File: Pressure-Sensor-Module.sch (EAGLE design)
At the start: 18 parts, among them IC1 ATTINY85

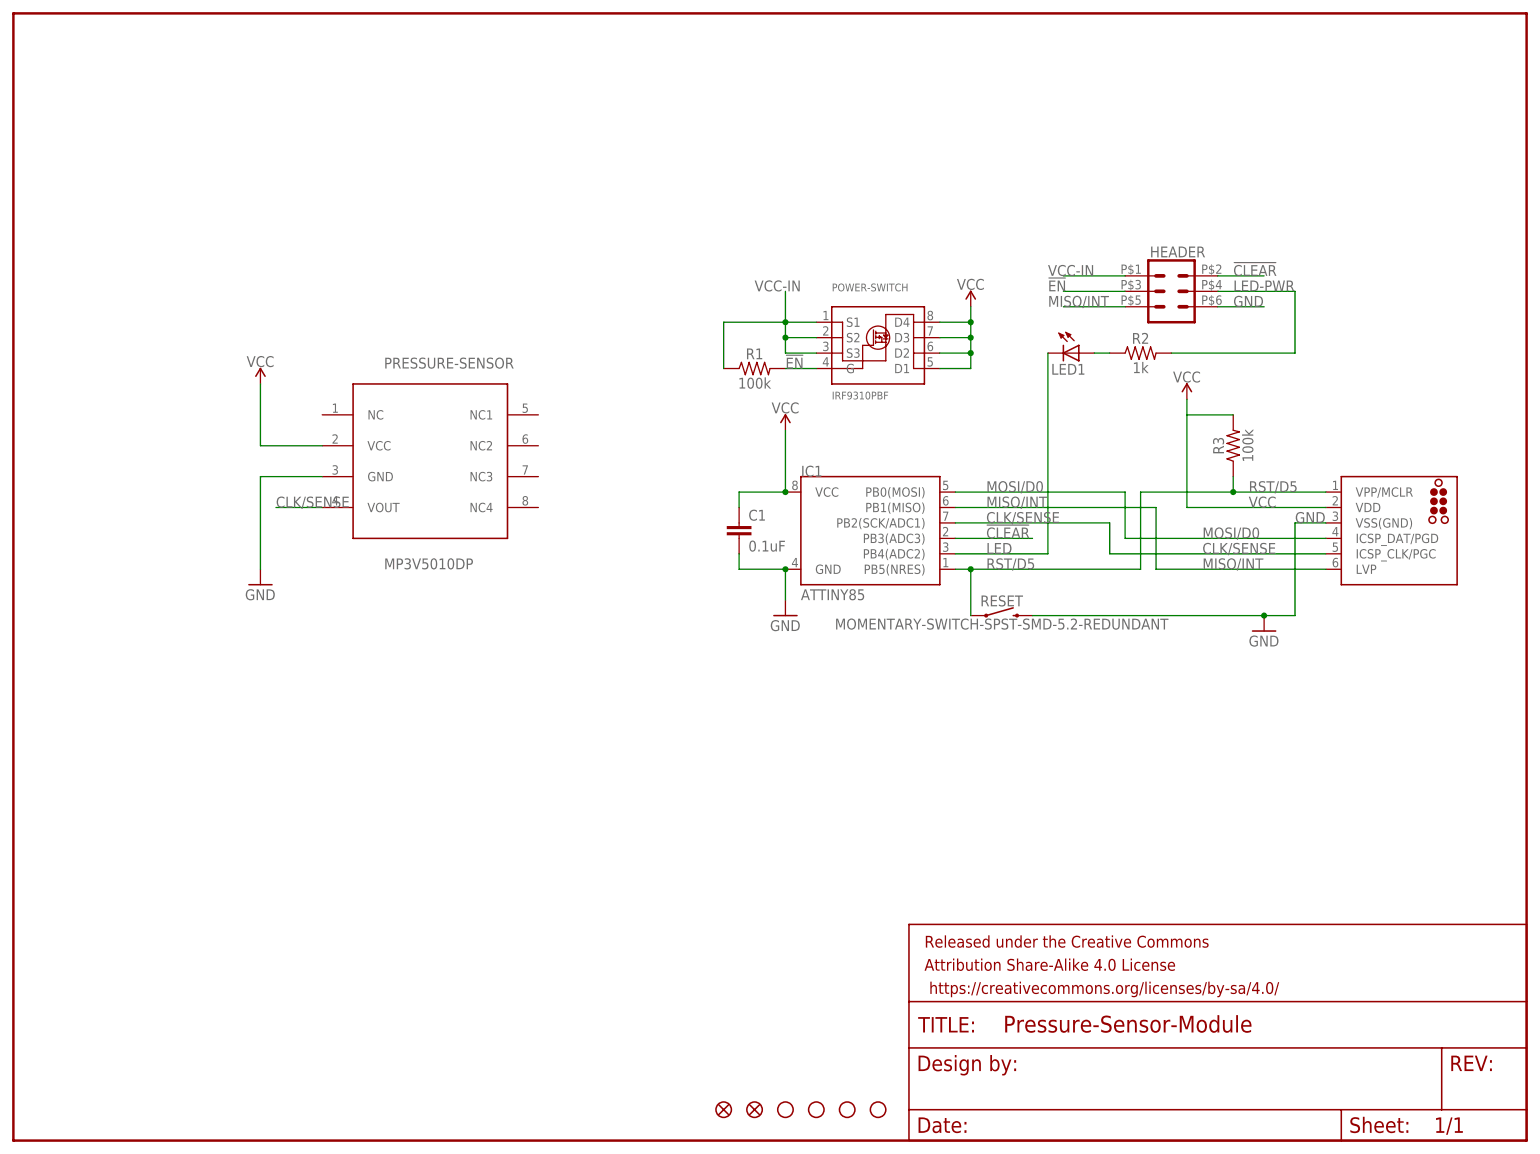
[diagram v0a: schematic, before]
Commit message: v2.0 Release Candidate
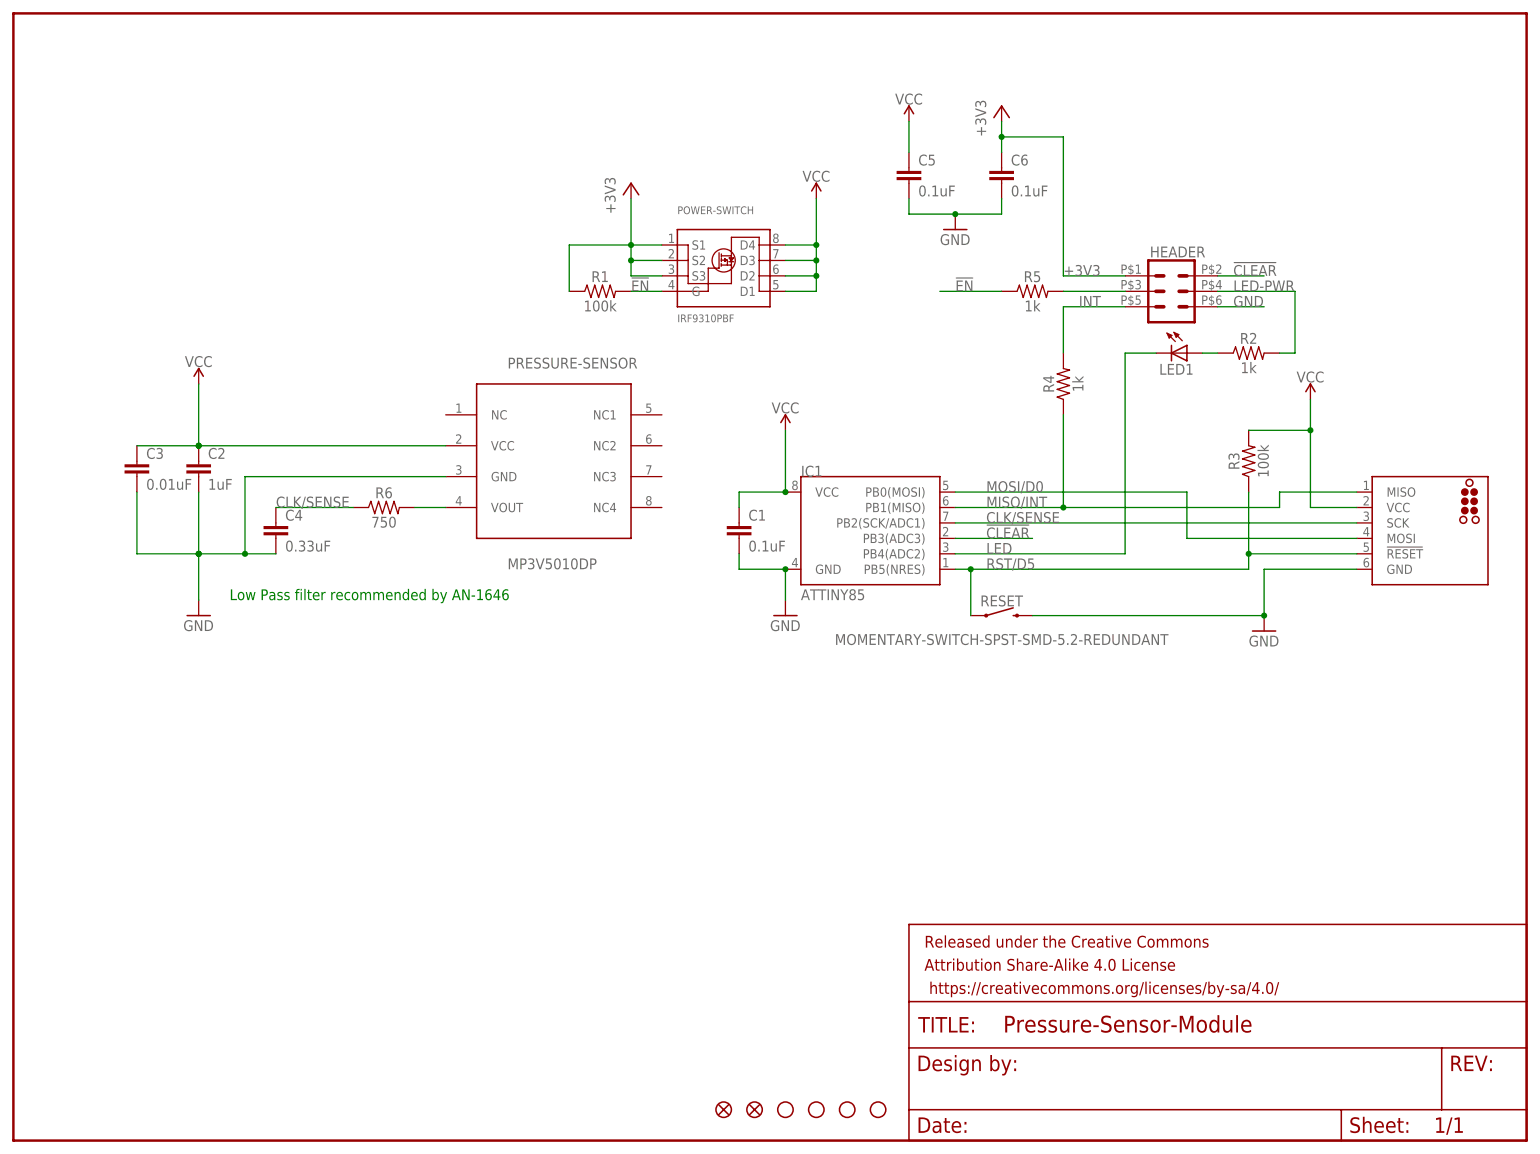
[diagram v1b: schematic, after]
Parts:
- added C2: 1uF, SparkFun-Capacitors:1.0UF-0805-25V-10%
- added C3: 0.01uF, SparkFun-Capacitors:1.0UF-0805-25V-10%
- added C4: 0.33uF, SparkFun-Capacitors:1.0UF-0805-25V-10%
- added C5, C6: 0.1uF, SparkFun-Capacitors:1.0UF-0805-25V-10%
- added R4, R5: 1k, SparkFun-Resistors:0.3OHM-0805-1/8W-1%
- added R6: 750, SparkFun-Resistors:0.3OHM-0805-1/8W-1%
- ICSP: device tag-connect:TC2030 -> tag-connect:TC2030-MCP-NL
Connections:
- removed net VCC-IN: HEADER.1, POWER-SWITCH.S1, POWER-SWITCH.S2, POWER-SWITCH.S3, R1.1
- new net +3V3: C6.1, HEADER.1, POWER-SWITCH.S1, POWER-SWITCH.S2, POWER-SWITCH.S3, R1.1
- new net INT: HEADER.5, R4.2
- new net N$2: HEADER.3, R5.2
- new net N$3: PRESSURE-SENSOR.VOUT, R6.2
- net !EN!: now also R5.1; no longer HEADER.3
- net CLK/SENSE: now also C4.1, ICSP.SCK, R6.1; no longer ICSP.ICSP_CLK/PGC, PRESSURE-SENSOR.VOUT
- net GND: now also C2.2, C3.2, C4.2, C5.2, C6.2, ICSP.GND; no longer ICSP.VSS(GND)
- net MISO/INT: now also ICSP.MISO, R4.1; no longer HEADER.5, ICSP.LVP
- net MOSI/D0: now also ICSP.MOSI; no longer ICSP.ICSP_DAT/PGD
- net RST/D5: now also ICSP.!RESET; no longer ICSP.VPP/MCLR
- net VCC: now also C2.1, C3.1, C5.1, ICSP.VCC; no longer ICSP.VDD
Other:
- note added: "Low Pass filter recommended by AN-1646"
- moved on the sheet: LED1, POWER-SWITCH, PRESSURE-SENSOR, R1, R2, R3
